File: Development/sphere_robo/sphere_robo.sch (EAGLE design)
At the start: 1 part, among them U1 RN4020-V/RM123

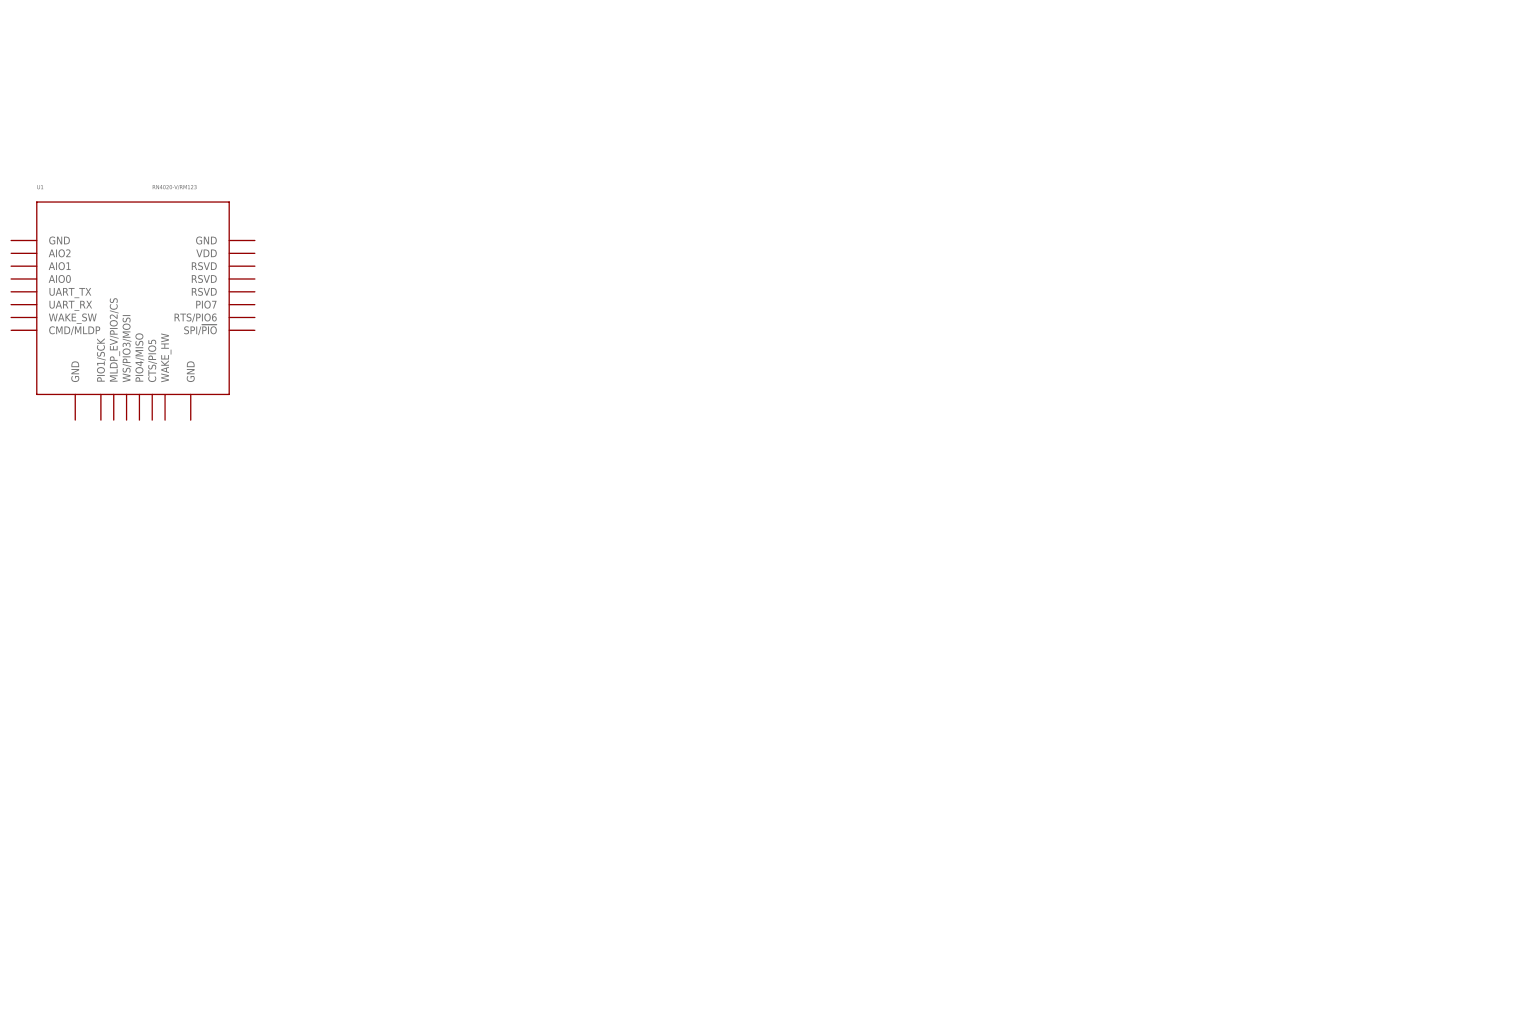
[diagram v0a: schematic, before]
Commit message: sphere_robo設計開始
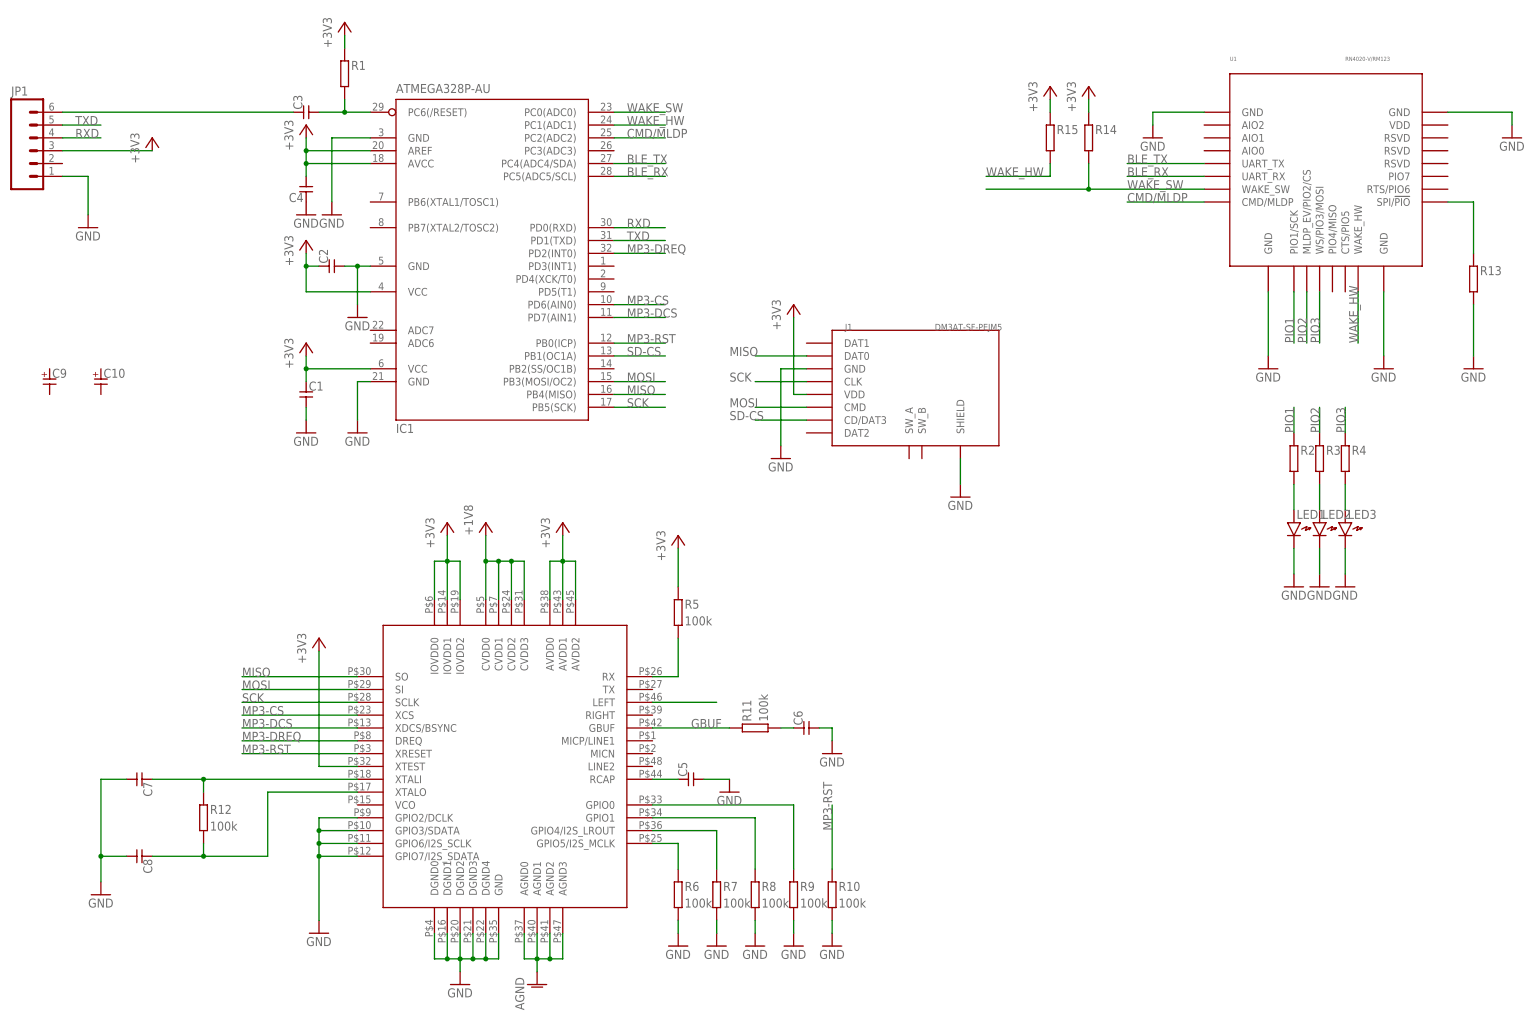
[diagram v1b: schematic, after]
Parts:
- added C1, C2, C3, C4, C5, C6, C7, C8: (no value), generic:CAPACITOR1608_REDUCED
- added C10, C9: (no value), generic:CAPACITOR-POLPANASONIC_D
- added IC1: ATMEGA328P-AU, AVR:ATMEGA328P-AU
- added J1: DM3AT-SF-PEJM5, SDcard:DM3AT-SF-PEJM5
- added JP1: (no value), header:M06NOSILK
- added LED1, LED2, LED3: (no value), generic:LED1608_REDUCED
- added R1, R13, R14, R15, R2, R3, R4: (no value), generic:RESISTOR1608_REDUCED
- added R10, R11, R12, R5, R6, R7, R8, R9: 100k, generic:RESISTOR1608_REDUCED
- added U$1: VS1053B, MP3:VS1053B
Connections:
- new net +1V8: U$1.CVDD0, U$1.CVDD1, U$1.CVDD2, U$1.CVDD3
- new net +3V3: C1.1, C2.1, C4.2, IC1.AREF, IC1.AVCC, IC1.VCC@1, IC1.VCC@2, J1.VDD, JP1.3, R1.1, R14.1, R15.1, R5.1, U$1.AVDD0, U$1.AVDD1, U$1.AVDD2, U$1.IOVDD0, U$1.IOVDD1, U$1.IOVDD2, U$1.XTEST
- new net AGND: U$1.AGND0, U$1.AGND1, U$1.AGND2, U$1.AGND3
- new net BLE_RX: IC1.PC5(ADC5/SCL), U1.UART_RX
- new net BLE_TX: IC1.PC4(ADC4/SDA), U1.UART_TX
- new net CMD/MLDP: IC1.PC2(ADC2), U1.CMD/MLDP
- new net GBUF: R11.1, U$1.GBUF
- new net GND: C1.2, C2.2, C4.1, C5.2, C6.2, C7.2, C8.2, IC1.GND, IC1.GND@1, IC1.GND@2, J1.GND, J1.SHIELD, JP1.1, LED1.K, LED2.K, LED3.K, R10.2, R13.2, R6.2, R7.2, R8.2, R9.2, U$1.DGND0, U$1.DGND1, U$1.DGND2, U$1.DGND3, U$1.DGND4, U$1.GND, U$1.GPIO2/DCLK, U$1.GPIO3/SDATA, U$1.GPIO6/I2S_SCLK, U$1.GPIO7/I2S_SDATA, U1.GND@1, U1.GND@2, U1.GND@3, U1.GND@4
- new net MISO: IC1.PB4(MISO), J1.DAT0, U$1.SO
- new net MOSI: IC1.PB3(MOSI/OC2), J1.CMD, U$1.SI
- new net MP3-CS: IC1.PD6(AIN0), U$1.XCS
- new net MP3-DCS: IC1.PD7(AIN1), U$1.XDCS/BSYNC
- new net MP3-DREQ: IC1.PD2(INT0), U$1.DREQ
- new net MP3-RST: IC1.PB0(ICP), R10.1, U$1.XRESET
- new net N$1: C3.2, IC1.PC6(/RESET), R1.2
- new net N$10: C5.1, U$1.RCAP
- new net N$11: R13.1, U1.SPI/!PIO
- new net N$12: R5.2, U$1.RX
- new net N$13: U$1.LEFT
- new net N$15: C7.1, R12.1, U$1.XTALI
- new net N$17: C6.1, R11.2
- new net N$19: C8.1, R12.2, U$1.XTALO
- new net N$2: C3.1, JP1.6
- new net N$3: LED1.A, R2.2
- new net N$4: LED2.A, R3.2
- new net N$5: LED3.A, R4.2
- new net N$6: R6.1, U$1.GPIO5/I2S_MCLK
- new net N$7: R7.1, U$1.GPIO4/I2S_LROUT
- new net N$8: R8.1, U$1.GPIO1
- new net N$9: R9.1, U$1.GPIO0
- new net PIO1: R2.1, U1.PIO1/SCK
- new net PIO2: R3.1, U1.MLDP_EV/PIO2/CS
- new net PIO3: R4.1, U1.WS/PIO3/MOSI
- new net RXD: IC1.PD0(RXD), JP1.4
- new net SCK: IC1.PB5(SCK), J1.CLK, U$1.SCLK
- new net SD-CS: IC1.PB1(OC1A), J1.CD/DAT3
- new net TXD: IC1.PD1(TXD), JP1.5
- new net WAKE_HW: IC1.PC1(ADC1), R15.2, U1.WAKE_HW
- new net WAKE_SW: IC1.PC0(ADC0), R14.2, U1.WAKE_SW
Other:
- moved on the sheet: U1
